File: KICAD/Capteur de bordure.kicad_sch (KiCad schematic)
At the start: 12 parts, among them J301 Conn_01x09, J302 Conn_01x09, J303 Conn_01x09

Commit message: update schematics
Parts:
- C301, C302, C303, C304, C305, C306: footprint (none) -> Capacitor_SMD:C_0603_1608Metric
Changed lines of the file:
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@@
       (effects (font (size 1.27 1.27)) (justify left))
     )
-    (property "Footprint" "" (at 46.99 93.98 0)
+    (property "Footprint" "Capacitor_SMD:C_0603_1608Metric" (at 46.99 93.98 0)
       (effects (font (size 1.27 1.27)) hide)
     )
@@
       (effects (font (size 1.27 1.27)) (justify left))
     )
-    (property "Footprint" "" (at 36.83 137.16 0)
+    (property "Footprint" "Capacitor_SMD:C_0603_1608Metric" (at 36.83 137.16 0)
       (effects (font (size 1.27 1.27)) hide)
     )
@@
       (effects (font (size 1.27 1.27)) (justify left))
     )
-    (property "Footprint" "" (at 36.83 99.06 0)
+    (property "Footprint" "Capacitor_SMD:C_0603_1608Metric" (at 36.83 99.06 0)
       (effects (font (size 1.27 1.27)) hide)
     )
@@
       (effects (font (size 1.27 1.27)) (justify left))
     )
-    (property "Footprint" "" (at 46.99 132.08 0)
+    (property "Footprint" "Capacitor_SMD:C_0603_1608Metric" (at 46.99 132.08 0)
       (effects (font (size 1.27 1.27)) hide)
     )
@@
       (effects (font (size 1.27 1.27)) (justify left))
     )
-    (property "Footprint" "" (at 46.99 168.91 0)
+    (property "Footprint" "Capacitor_SMD:C_0603_1608Metric" (at 46.99 168.91 0)
       (effects (font (size 1.27 1.27)) hide)
     )
@@
       (effects (font (size 1.27 1.27)) (justify left))
     )
-    (property "Footprint" "" (at 36.83 173.99 0)
-      (effects (font (size 1.27 1.27)) hide)
-    )
+    (property "Footprint" "Capacitor_SMD:C_0603_1608Metric" (at 36.83 173.99 0)
+      (effects (font (size 1.27 1.27)) hide)
+    )

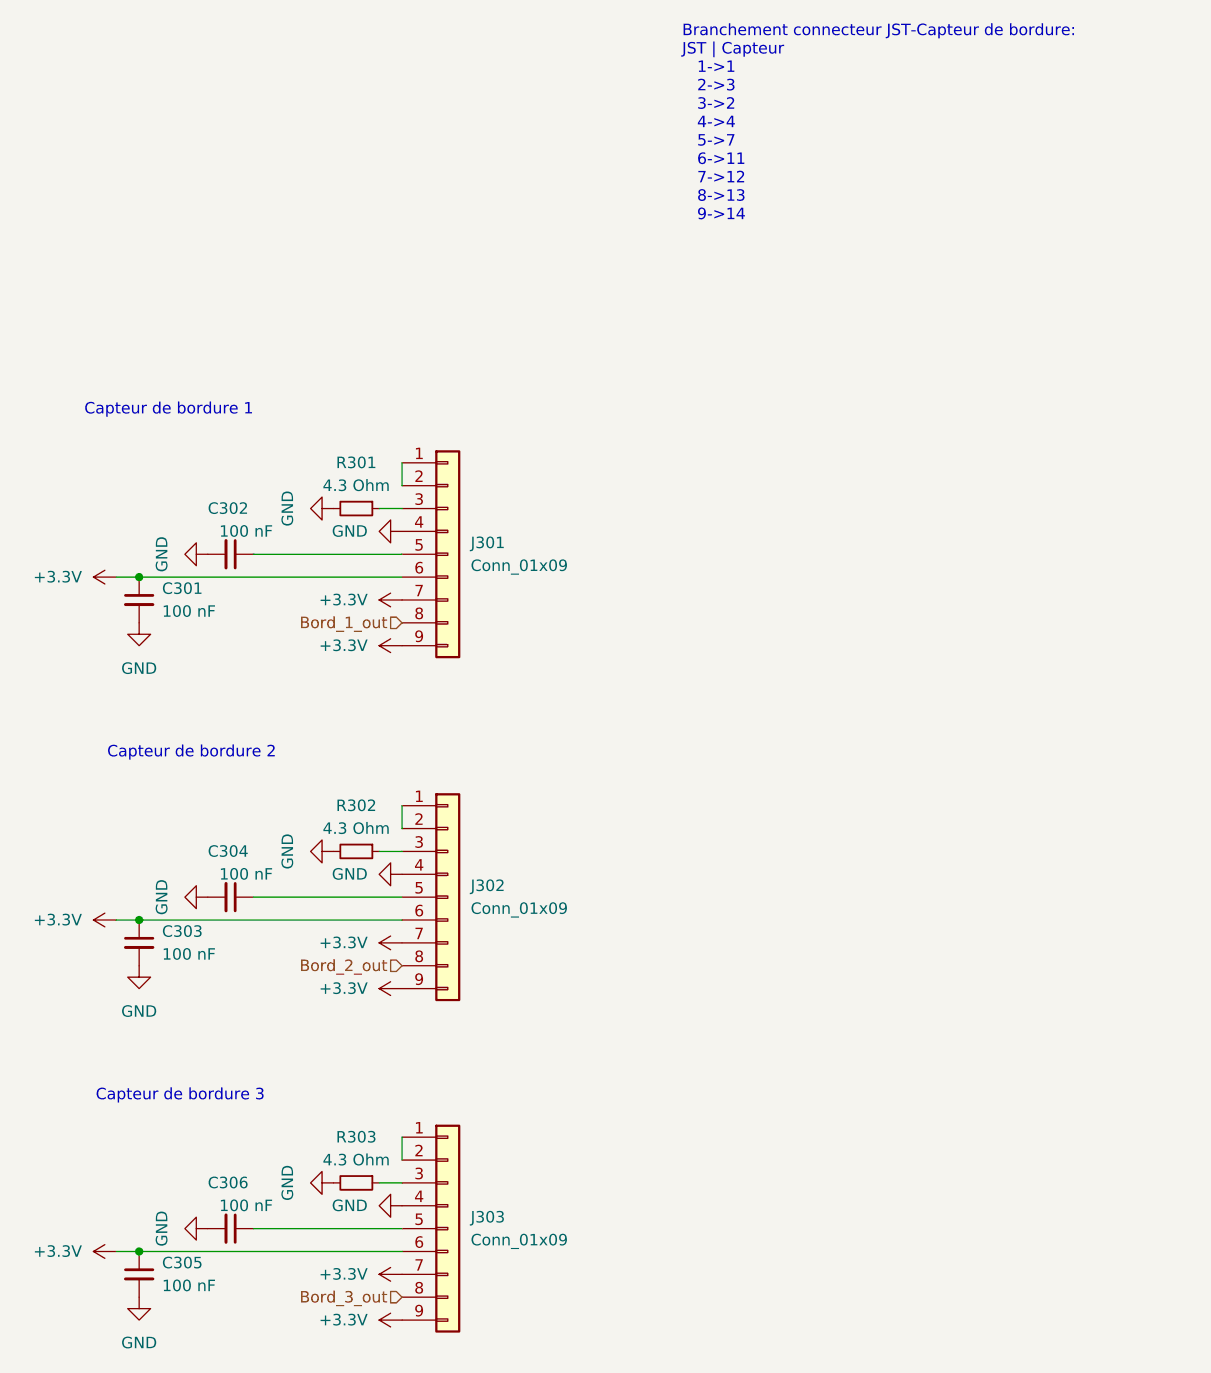
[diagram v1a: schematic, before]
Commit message: Completed schematics
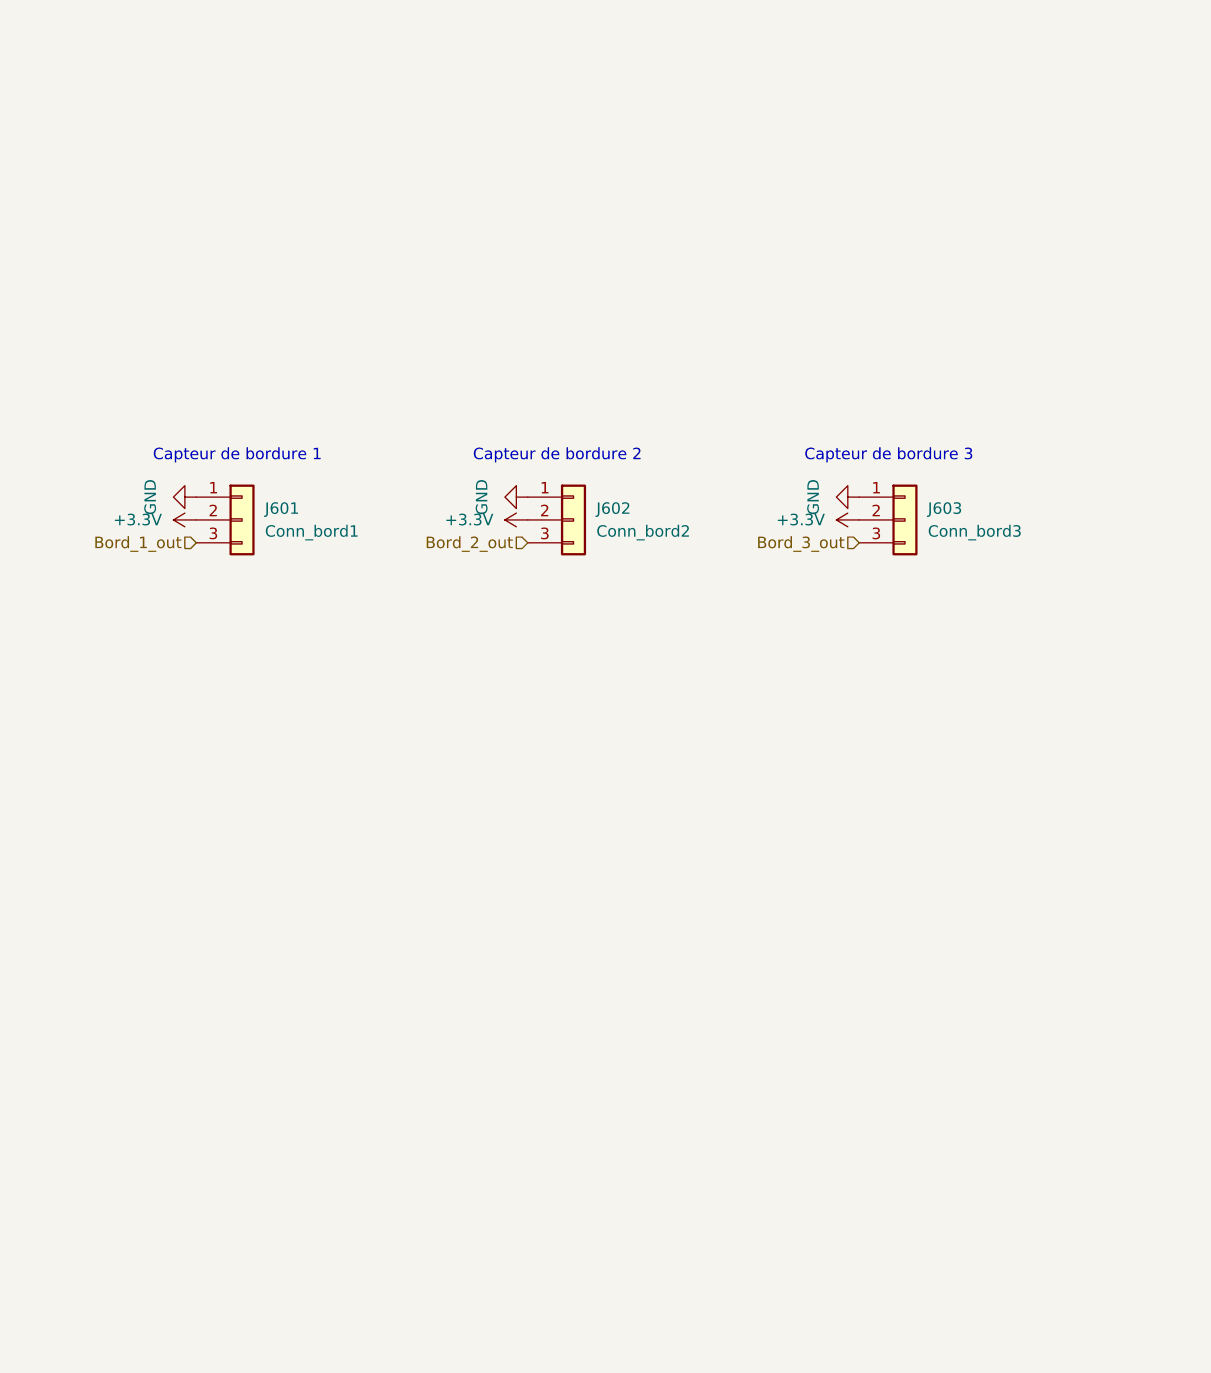
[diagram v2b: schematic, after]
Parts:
- removed C301, C302, C303, C304, C305, C306: 100 nF, Capacitor_SMD:C_0603_1608Metric, symbol Device:C_Small
- removed J301, J302, J303: Conn_01x09, symbol Connector_Generic:Conn_01x09
- removed R301, R302, R303: 4.3 Ohm, symbol Device:R_Small
- added J601: Conn_bord1, Connector_JST:JST_XH_S3B-XH-A_1x03_P2.50mm_Horizontal, symbol Connector_Generic:Conn_01x03
- added J602: Conn_bord2, Connector_JST:JST_XH_S3B-XH-A_1x03_P2.50mm_Horizontal, symbol Connector_Generic:Conn_01x03
- added J603: Conn_bord3, Connector_JST:JST_XH_S3B-XH-A_1x03_P2.50mm_Horizontal, symbol Connector_Generic:Conn_01x03
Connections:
- net +3.3V: now also J601.2 (Pin_2), J602.2 (Pin_2), J603.2 (Pin_2)
- net Bord_1_out: now also J601.3 (Pin_3)
- net Bord_2_out: now also J602.3 (Pin_3)
- net Bord_3_out: now also J603.3 (Pin_3)
- net GND: now also J601.1 (Pin_1), J602.1 (Pin_1), J603.1 (Pin_1)
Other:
- note removed: "Branchement connecteur JST-Capteur de bordure: JST | Capteur 1->1 2->3 3->2 4->4 5->7 6->11 7->12 8->13 9->14"
